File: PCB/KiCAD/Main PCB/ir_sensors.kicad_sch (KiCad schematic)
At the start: 35 parts, among them IC1 ADG608BRZ, IC2 ADG608BRZ, J7 Conn_02x03_Odd_Even, U3 ATmega328PB-A, Y1 Crystal

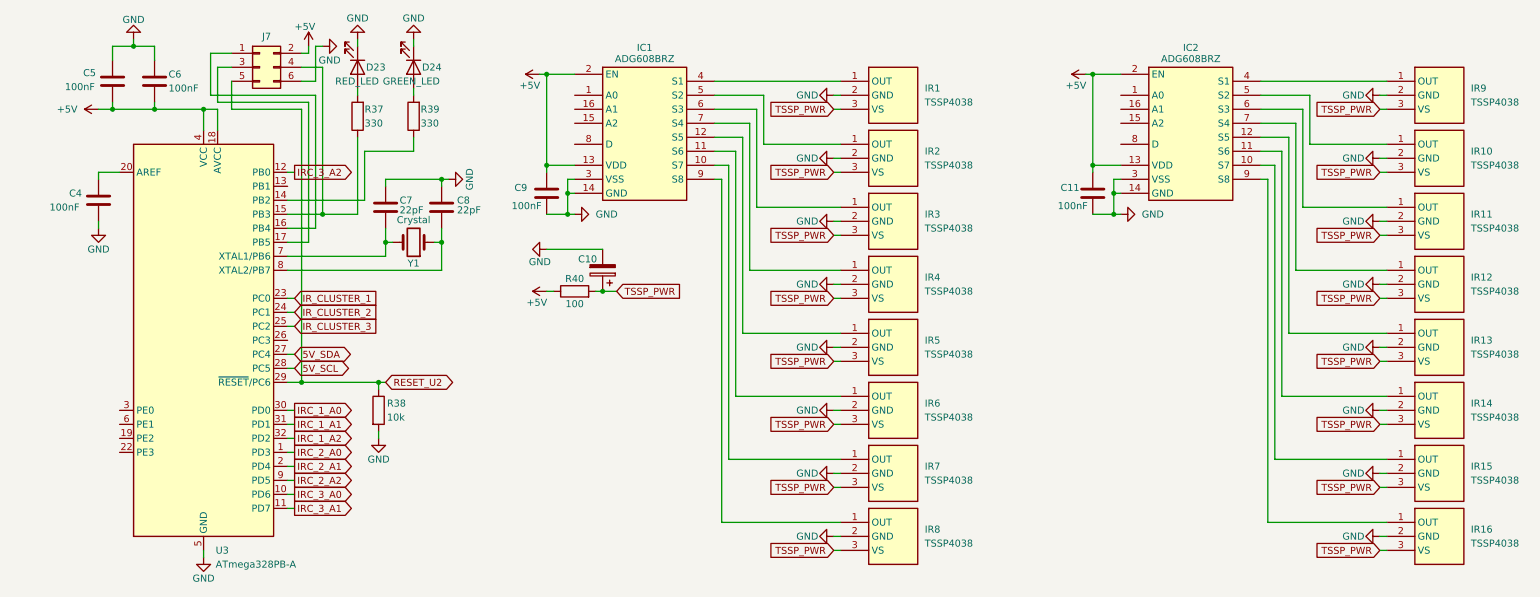
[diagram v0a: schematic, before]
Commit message: Changes to the main PCB
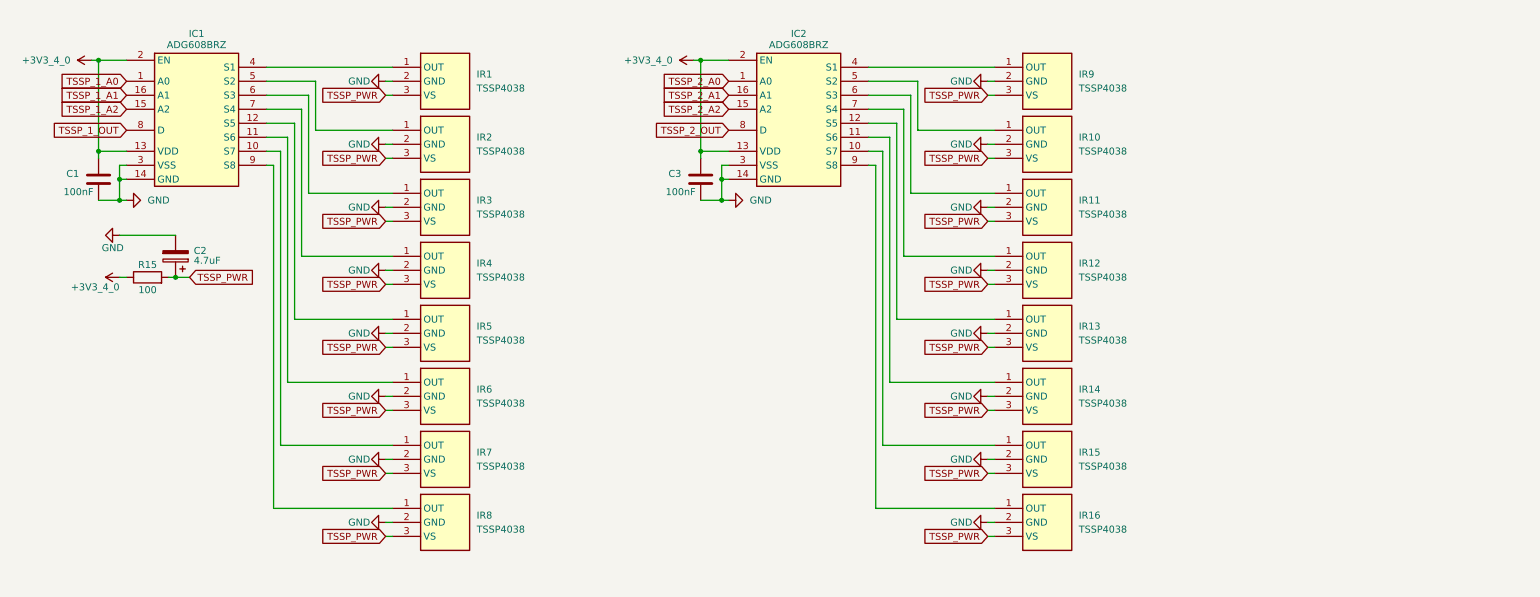
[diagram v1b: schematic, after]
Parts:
- removed C4, C5, C6: 100nF, Capacitor_SMD:C_0805_2012Metric_Pad1.18x1.45mm_HandSolder, symbol Device:C
- removed C7, C8: 22pF, Capacitor_SMD:C_0805_2012Metric_Pad1.18x1.45mm_HandSolder, symbol Device:C
- removed D23: RED_LED, LED_SMD:LED_0805_2012Metric_Pad1.15x1.40mm_HandSolder, symbol Device:LED
- removed D24: GREEN_LED, LED_SMD:LED_0805_2012Metric_Pad1.15x1.40mm_HandSolder, symbol Device:LED
- removed J7: Conn_02x03_Odd_Even, Connector_IDC:IDC-Header_2x03_P2.54mm_Vertical_SMD, symbol Connector_Generic:Conn_02x03_Odd_Even
- removed R37, R39: 330, Resistor_SMD:R_0805_2012Metric_Pad1.20x1.40mm_HandSolder, symbol Device:R
- removed R38: 10k, Resistor_SMD:R_0805_2012Metric_Pad1.20x1.40mm_HandSolder, symbol Device:R
- removed U3: ATmega328PB-A, Package_QFP:TQFP-32_7x7mm_P0.8mm, symbol MCU_Microchip_ATmega:ATmega328PB-A
- removed Y1: Crystal, Crystal:Crystal_SMD_HC49-SD, symbol Device:Crystal
- renumbered C9 to C1, C10 to C2, C11 to C3, R40 to R15
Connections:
- net TSSP_2_A0: now reaches IC2.1 (A0)
- net TSSP_2_A2: now reaches IC2.15 (A2)
- net TSSP_2_A1: now reaches IC2.16 (A1)
- net TSSP_2_OUT: now reaches IC2.8 (D)
- net TSSP_1_A0: now reaches IC1.1 (A0)
- net TSSP_1_A2: now reaches IC1.15 (A2)
- net TSSP_1_A1: now reaches IC1.16 (A1)
- net TSSP_1_OUT: now reaches IC1.8 (D)
- net +5V renamed +3V3_4_0
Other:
- moved on the sheet: C1, C2, C3, IC1, IC2, IR1, IR10, IR11, IR12, IR13, IR14, IR15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
